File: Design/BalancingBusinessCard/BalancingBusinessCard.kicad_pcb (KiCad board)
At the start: 2 copper layers, 51 x 89 mm, 31 parts, among them J101 TestPoints, M201 Motor_DC, U101 ATtiny261-20SU, U201 AP1017AEN, U401 LIS3DHTR, U501 FT440CA

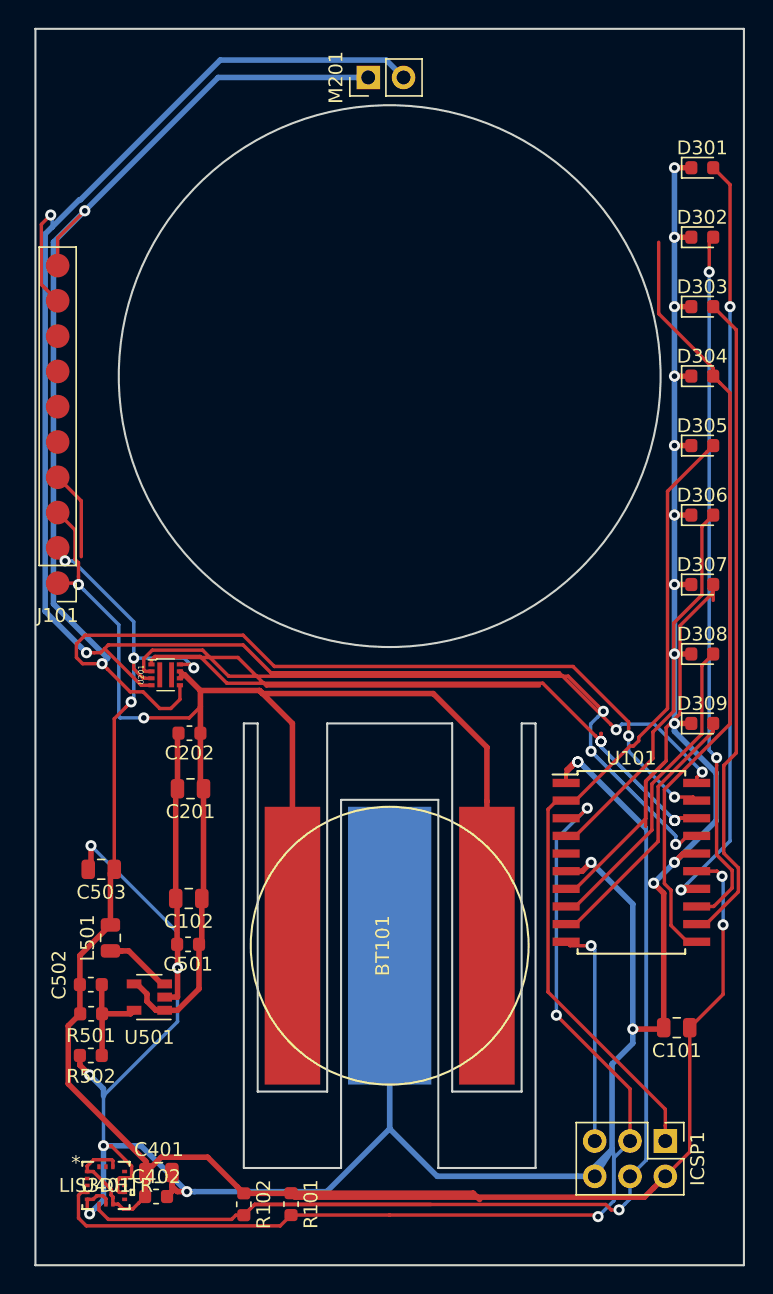
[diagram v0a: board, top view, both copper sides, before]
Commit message: Manual cleanup
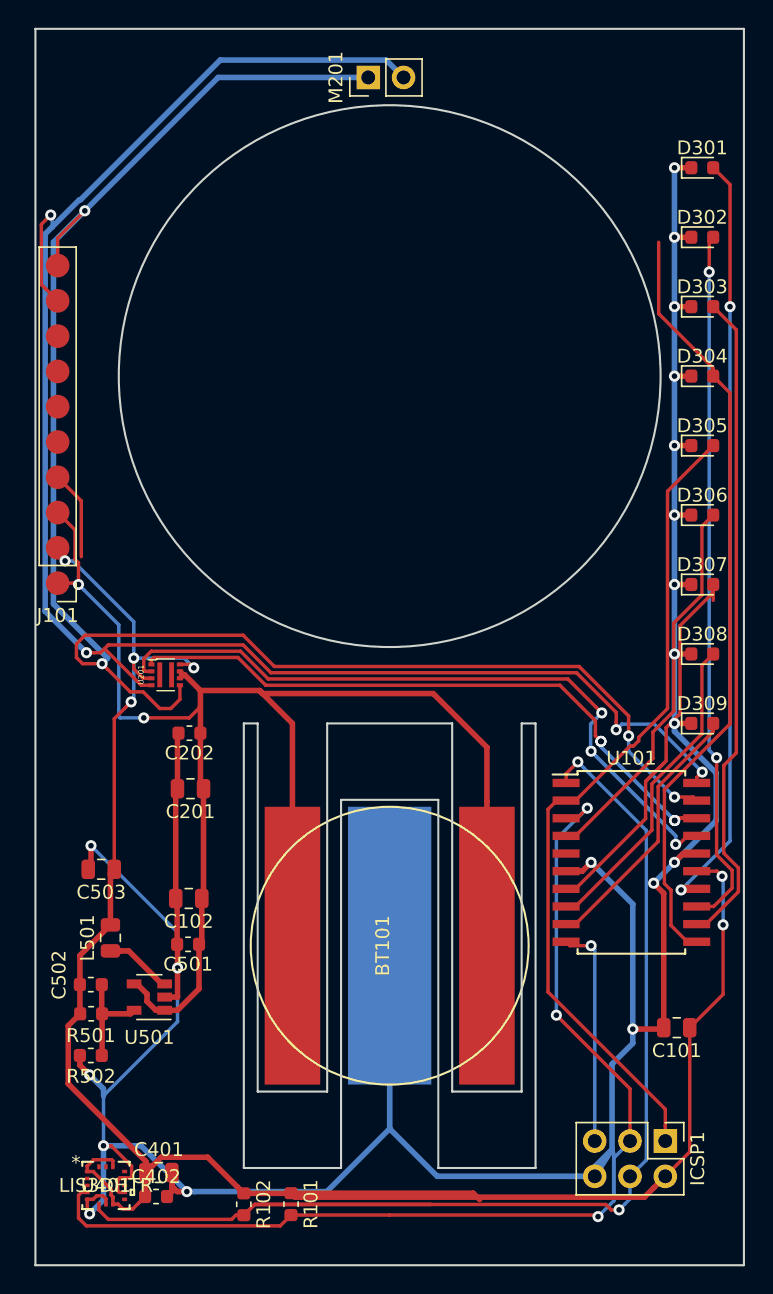
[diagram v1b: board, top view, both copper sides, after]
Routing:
- net /MOSI: track 122.6 -> 89.5 mm, vias 3 -> 2
- net /INA: track 83.6 -> 55.0 mm
- net /LED_6: track 32.4 -> 29.2 mm
- net /ADC0: track 124.8 -> 125.5 mm

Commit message: Automatic cleanup
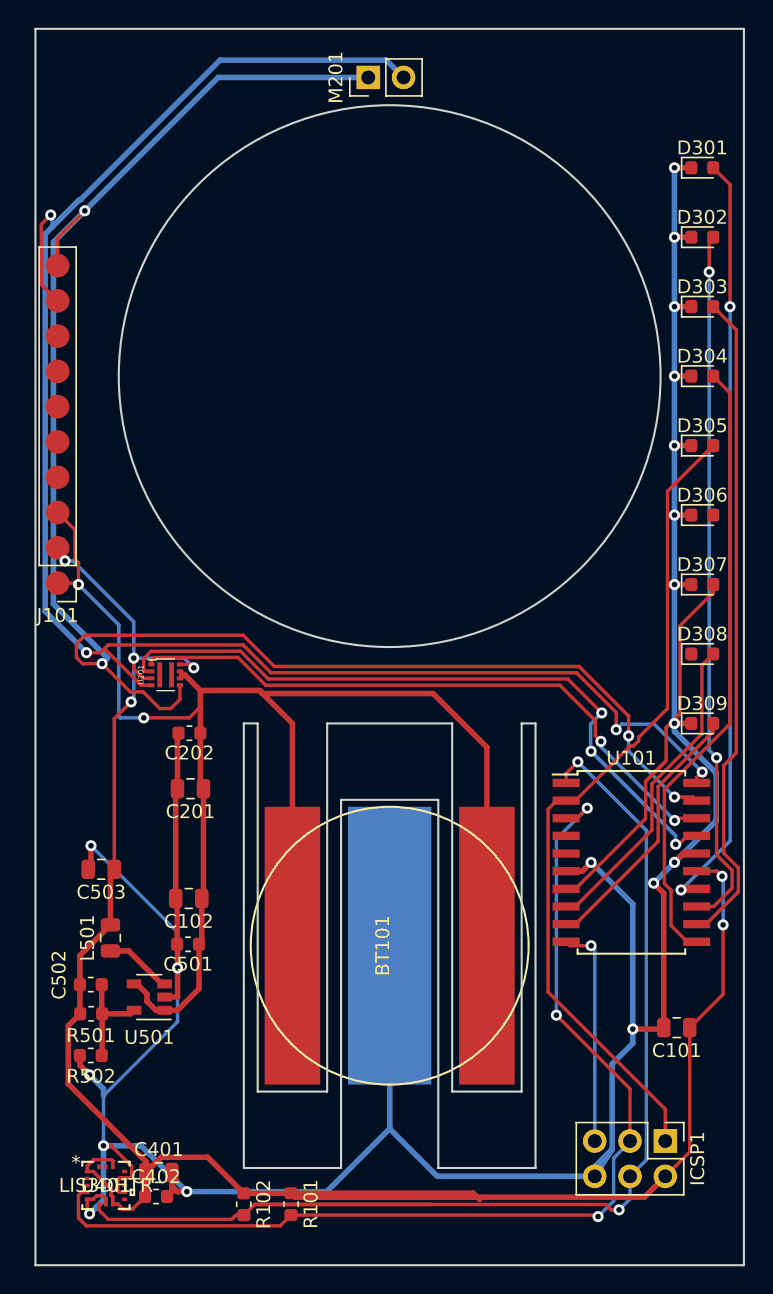
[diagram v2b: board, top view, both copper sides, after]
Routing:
- net /LED_5: track 27.9 -> 0.68 mm
- net /LED_3: track 55.8 -> 44.5 mm
- net /INA: track 55.0 -> 45.4 mm, vias 4 -> 2
- net /RESET: track 22.5 -> 16.1 mm
- net /SCK: track 79.1 -> 75.6 mm
- net GND: track 232.6 -> 231.4 mm, vias 19 -> 18
- net /MOSI: track 89.5 -> 88.4 mm
- net /LED_6: track 29.2 -> 28.6 mm

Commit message: Fixed routing
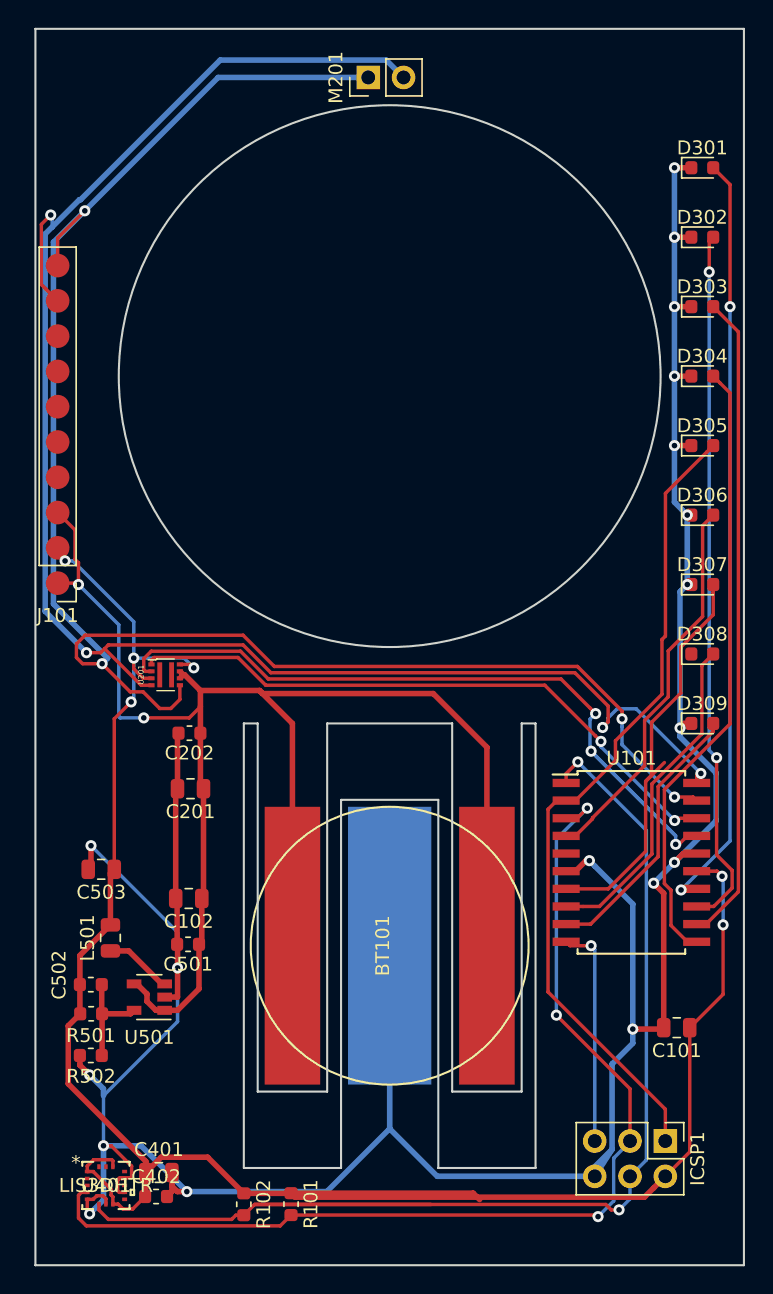
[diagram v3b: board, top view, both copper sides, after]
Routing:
- net /LED_5: track 0.68 -> 27.9 mm
- net /ADC0: track 125.5 -> 127.1 mm
- net GND: track 231.4 -> 229.8 mm
- net /LED_6: track 28.6 -> 30.0 mm
- net /LED_7: track 23.0 -> 24.0 mm
- net /LED_2: track 47.6 -> 46.8 mm
- net /LED_8: track 19.2 -> 19.9 mm
- net /INA: track 45.4 -> 44.8 mm
- net /INB: track 59.0 -> 58.4 mm
